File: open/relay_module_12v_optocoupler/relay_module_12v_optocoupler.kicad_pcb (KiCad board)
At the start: 2 copper layers, 30.2 x 71.1 mm, 15 parts, among them J1 Conn_01x02_Pin, J2 Conn_01x03_Pin, K1 Relay_SPDT, Q1 BC337, U1 PC817

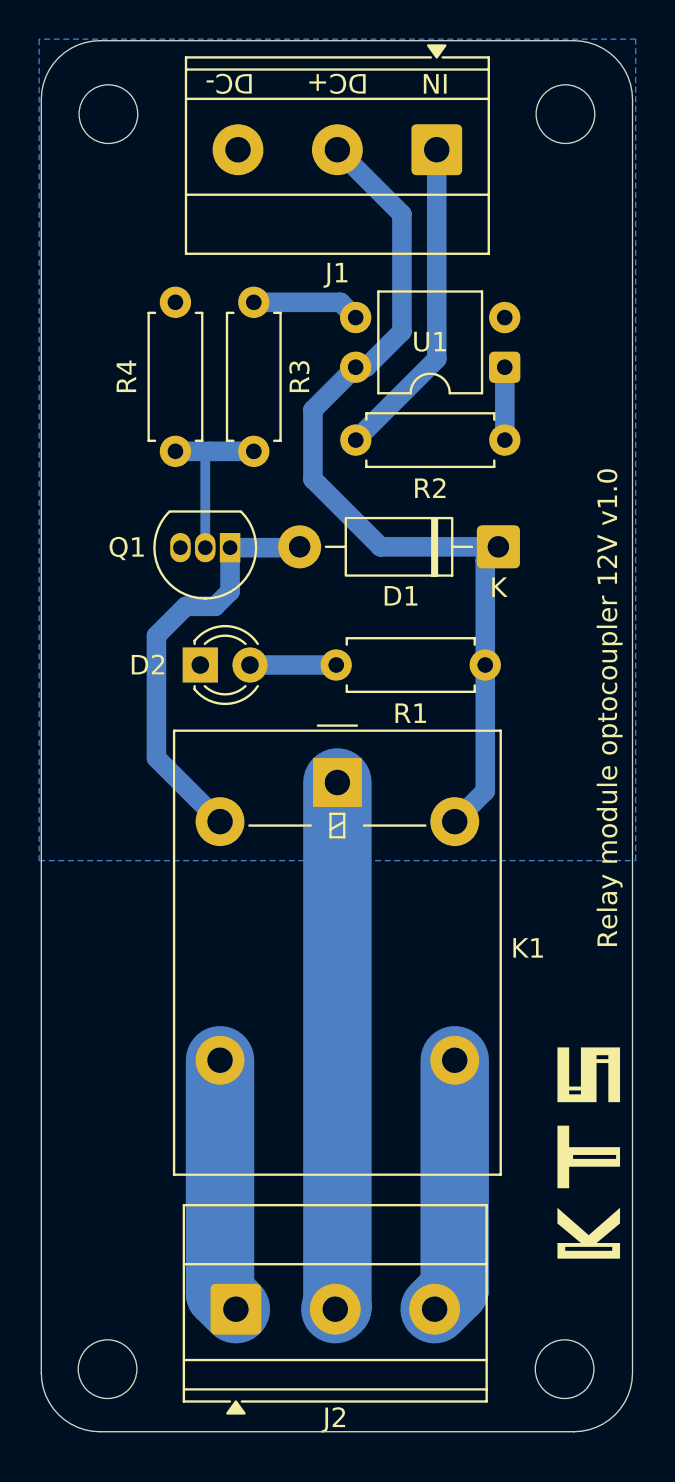
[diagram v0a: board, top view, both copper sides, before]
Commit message: v1.0.0
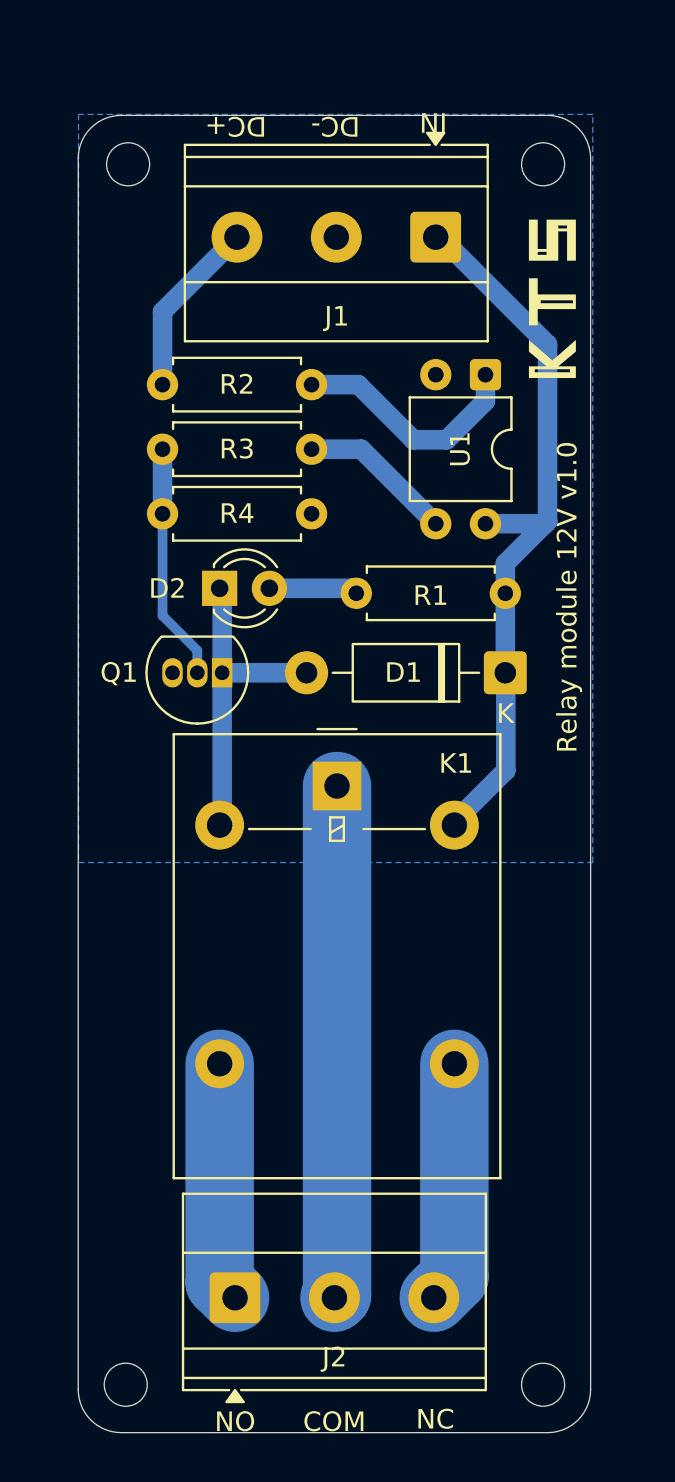
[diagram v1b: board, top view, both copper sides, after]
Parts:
- removed the REF** at (160.9, 72.8)
- removed the REF** at (137.5, 137.0)
- removed the REF** at (137.5, 72.8)
- removed the REF** at (160.9, 137.0)
- added REF**: MountingHole_2.2mm_M2, MountingHole:MountingHole_2.2mm_M2, F.Cu at (159.8, 137.8)
- added REF**: MountingHole_2.2mm_M2, MountingHole:MountingHole_2.2mm_M2, F.Cu at (159.8, 75.4)
- added REF**: MountingHole_2.2mm_M2, MountingHole:MountingHole_2.2mm_M2, F.Cu at (138.4, 137.8)
- added REF**: MountingHole_2.2mm_M2, MountingHole:MountingHole_2.2mm_M2, F.Cu at (138.6, 75.4)
- moved R4 12.9 mm to (147.9, 93.3), turned to 180 degrees
- moved R2 10.3 mm to (140.3, 86.7)
- moved R3 8.07 mm to (147.9, 90.0), turned to 180 degrees
- moved D1 6.45 mm to (157.8, 101.4)
- moved Q1 6.41 mm to (143.4, 101.4)
- moved J1 4.47 mm to (154.3, 79.1)
- moved D2 4.04 mm to (143.2, 97.1)
- moved R1 3.81 mm to (157.8, 97.3)
- moved U1 1.06 mm to (156.8, 86.2), turned to -90 degrees
- moved J2 0.59 mm to (144.0, 133.3)
- moved K1 0.18 mm to (149.2, 107.2)
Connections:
- D2 pad 1: GND -> Net-(D1-A)
- J1 pad 1: Net-(J1-Pin_1) -> Net-(D1-K)
- J1 pad 2: Net-(D1-K) -> GND
- J1 pad 3: GND -> Net-(J1-Pin_3)
- R2 pad 1: Net-(J1-Pin_1) -> Net-(J1-Pin_3)
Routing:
- net Net-(J1-Pin_1): track 16.6 -> 0.00 mm
- net Net-(J1-Pin_3): track 0.00 -> 9.11 mm
- net Net-(D1-K): track 46.4 -> 37.9 mm
- net Net-(R2-Pad2): track 3.73 -> 12.2 mm
- net Net-(D1-A): track 21.4 -> 16.8 mm
- net Net-(Q1-B): track 9.03 -> 12.1 mm
- net Net-(R3-Pad1): track 5.53 -> 7.93 mm
- net NO_1: track 13.1 -> 12.3 mm
- net C_1: track 27.0 -> 26.2 mm
- net NC_1: track 13.2 -> 12.4 mm
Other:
- board size 30.2 x 71.1 mm -> 26.2 x 67.3 mm
- board text added: "COM"
- board text added: "NC"
- board text added: "NO"
- board text added: "Relay module 12V v1.0"
- board text removed: "Relay module optocoupler 12V v1.0"
